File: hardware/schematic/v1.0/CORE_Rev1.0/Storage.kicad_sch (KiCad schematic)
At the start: 43 parts, among them J12 USB_C_Receptacle_USB2.0_16P, U1 TXS02612RTWR, U3 FT2232HL, U6 93LC56BT-I_OT, X1 X322512MSB4SI

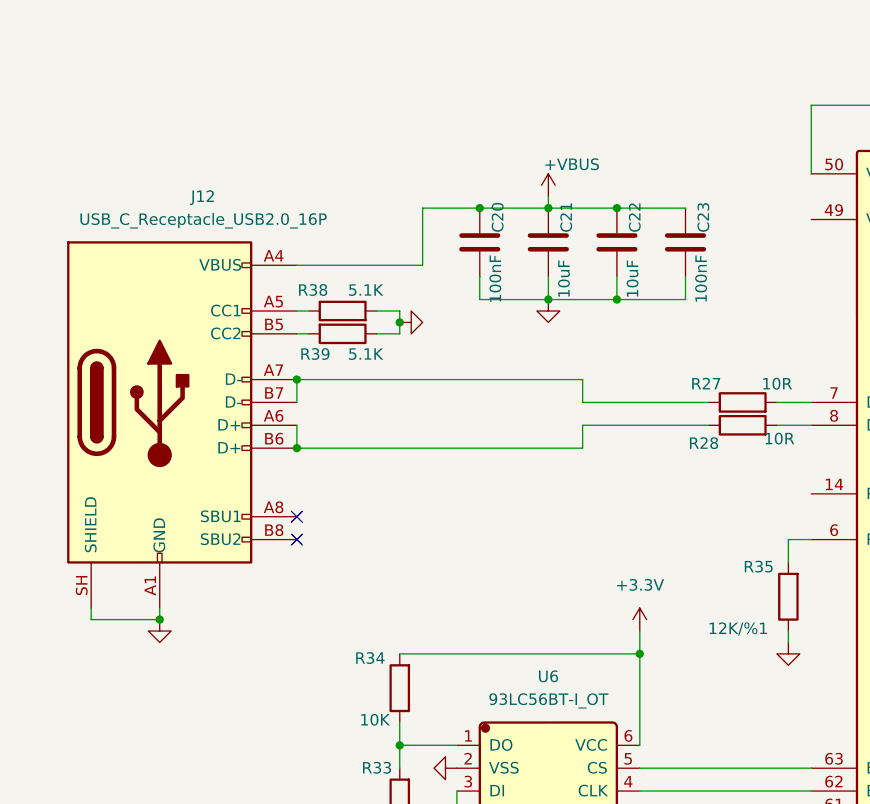
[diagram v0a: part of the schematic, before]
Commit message: sch update
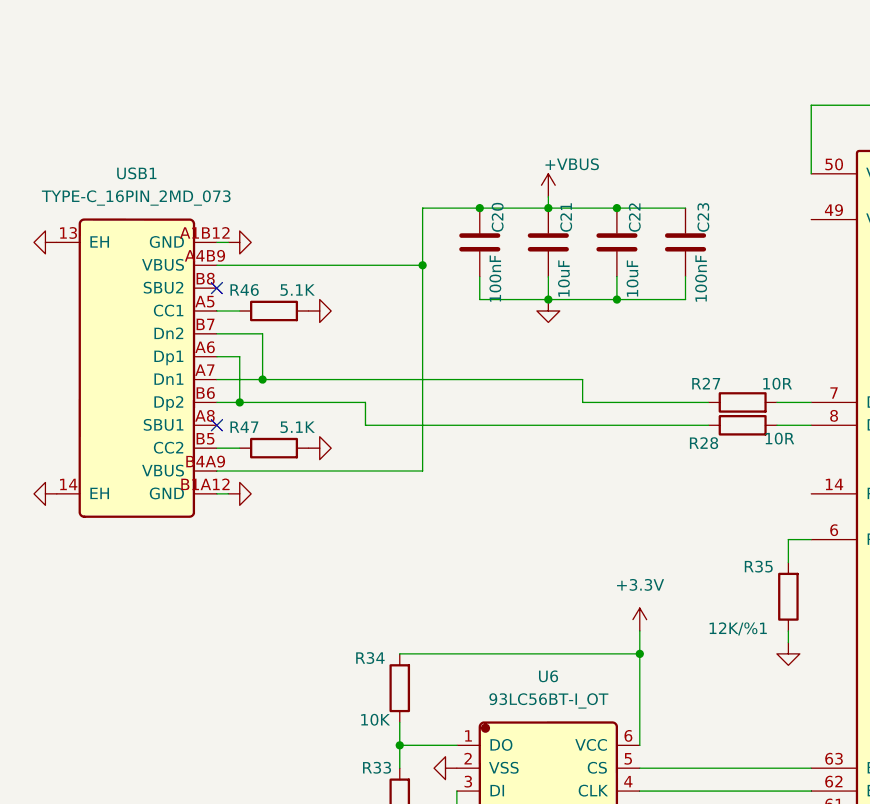
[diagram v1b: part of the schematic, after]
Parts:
- removed J12: USB_C_Receptacle_USB2.0_16P, Connector_USB:USB_C_Receptacle_Palconn_UTC16-G, symbol Connector:USB_C_Receptacle_USB2.0_16P
- removed R38, R39: 5.1K, Resistor_SMD:R_0402_1005Metric, symbol Device:R
- added R46, R47: 5.1K, Resistor_SMD:R_0402_1005Metric, symbol Device:R
- added USB1: TYPE-C_16PIN_2MD_073, CORE:TYPE-C_16PIN_2MD_073, symbol CORE:TYPE-C_16PIN_2MD_073
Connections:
- net +VBUS: now also USB1.A4B9 (VBUS), USB1.B4A9 (VBUS)
- net GND: now also R46.2, R47.2, USB1.13 (EH), USB1.14 (EH), USB1.A1B12 (GND), USB1.B1A12 (GND)
- net at R28.1: now also USB1.A6 (Dp1), USB1.B6 (Dp2)
- net at R27.1: now also USB1.A7 (Dn1), USB1.B7 (Dn2)
- new net: R46.1, USB1.A5 (CC1)
- new net: R47.1, USB1.B5 (CC2)

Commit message: sch update
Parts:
- C2, C20, C23, C24, C25, C3, C4, C5: footprint Capacitor_SMD:C_0402_1005Metric -> CORE:C_0402_1005Metric; symbol Device:C -> CORE:C
- C21, C22: footprint Capacitor_SMD:C_0603_1608Metric -> CORE:C_0603_1608Metric; symbol Device:C -> CORE:C
- R11, R12, R13, R14, R15, R16, R17, R18, R19, R20, R21, R22, R23, R27, R28, R29, R30, R31, R32, R33, R34, R35, R43, R44, R46, R47: footprint Resistor_SMD:R_0402_1005Metric -> CORE:R_0402_1005Metric; symbol Device:R -> CORE:R
